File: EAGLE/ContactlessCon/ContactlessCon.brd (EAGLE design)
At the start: 57.1 x 31.4 mm, 5 parts, among them J1 PINHEADER-212*1, J2 PINHEADER-818*1, X1 0446200002

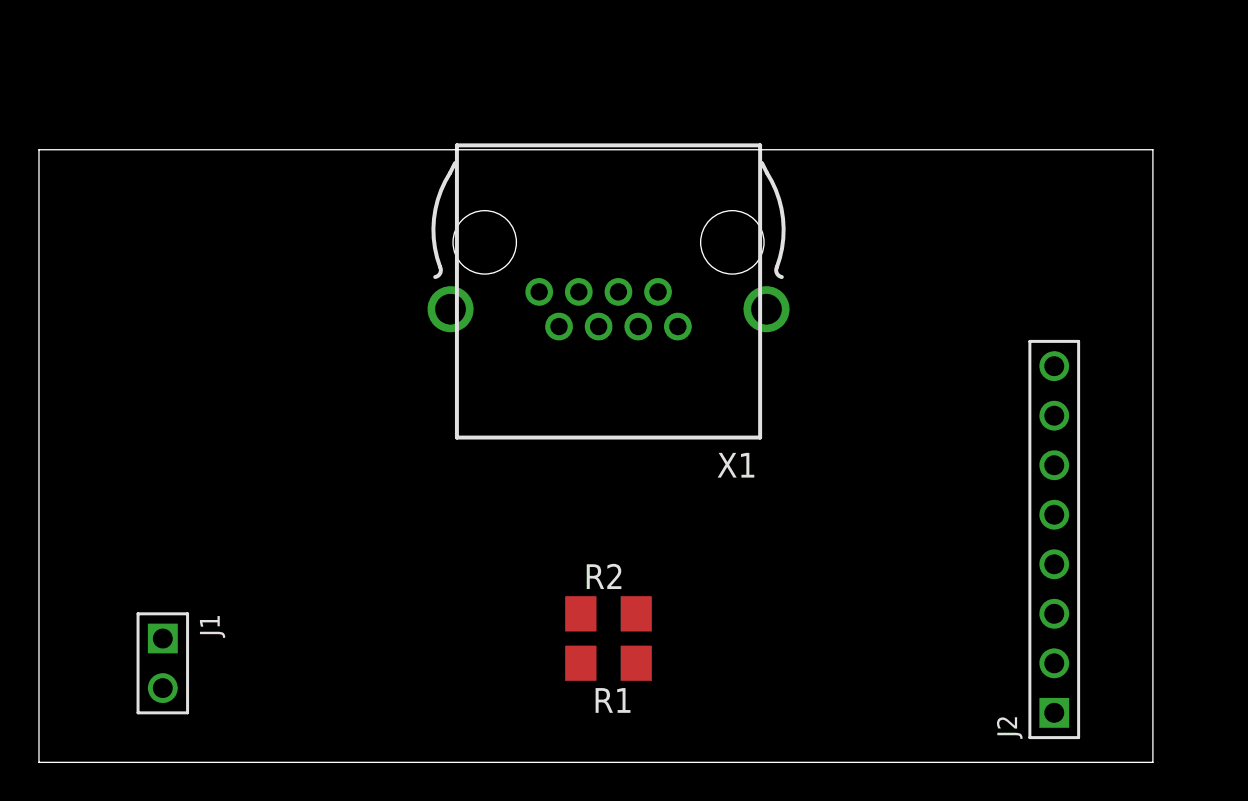
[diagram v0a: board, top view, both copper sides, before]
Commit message: Conの配線終了
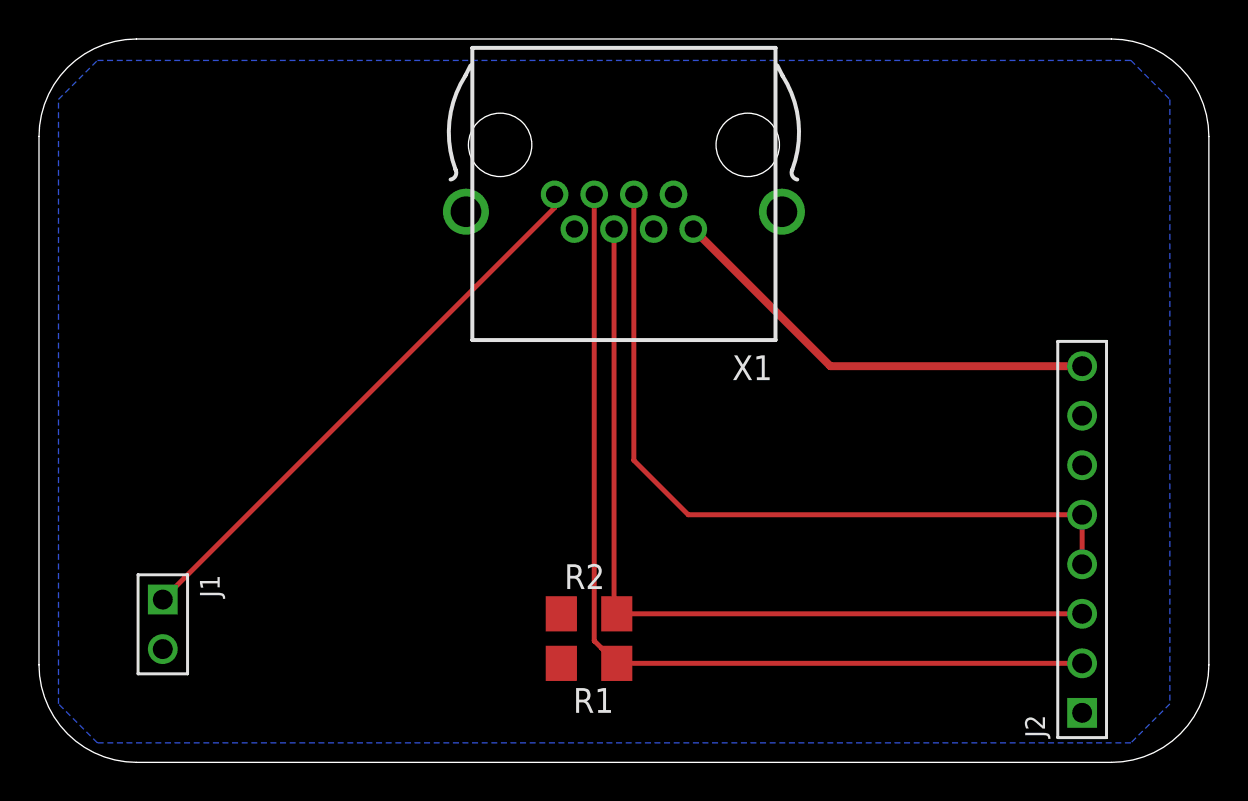
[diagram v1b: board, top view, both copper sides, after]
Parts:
- moved X1 5.06 mm to (30.0, 31.7)
- moved J1 2.00 mm to (6.35, 7.08)
- moved J2 1.43 mm to (53.5, 8.89)
- moved R1 1.00 mm to (28.2, 5.08)
- moved R2 1.00 mm to (28.2, 7.62)
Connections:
- net GPIO: now also X1.5; no longer X1.3
- net SCL: now also X1.4; no longer X1.5
- net SDA: now also X1.3; no longer X1.4
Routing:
- net SDA: track 0.00 -> 48.4 mm
- net SCL: track 0.00 -> 44.0 mm
- net GPIO: track 0.00 -> 40.3 mm
- net SPEAKER: track 0.00 -> 29.1 mm
- net +3V3: track 0.00 -> 22.9 mm
- added copper zone on layer 16, net GND
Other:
- board size 57.1 x 31.4 mm -> 60 x 37.1 mm
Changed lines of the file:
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@@
 <board>
 <plain>
-<wire x1="0" y1="0" x2="57.13" y2="0" width="0" layer="20"/>
-<wire x1="57.13" y1="0" x2="57.13" y2="31.42" width="0" layer="20"/>
-<wire x1="57.13" y1="31.42" x2="0" y2="31.42" width="0" layer="20"/>
-<wire x1="0" y1="31.42" x2="0" y2="0" width="0" layer="20"/>
+<wire x1="0" y1="32.1" x2="0" y2="5" width="0" layer="20"/>
+<wire x1="0" y1="5" x2="5" y2="0" width="0" layer="20" curve="90"/>
+<wire x1="5" y1="0" x2="55" y2="0" width="0" layer="20"/>
+<wire x1="55" y1="0" x2="60" y2="5" width="0" layer="20" curve="90"/>
+<wire x1="60" y1="5" x2="60" y2="32.1" width="0" layer="20"/>
+<wire x1="60" y1="32.1" x2="55" y2="37.1" width="0" layer="20" curve="90"/>
+<wire x1="55" y1="37.1" x2="5" y2="37.1" width="0" layer="20"/>
+<wire x1="5" y1="37.1" x2="0" y2="32.1" width="0" layer="20" curve="90"/>
 </plain>
 <attributes>
@@
 </autorouter>
 <elements>
-<element name="J1" library="PINHEADER" package="PINHEADER-2*1" value="PINHEADER-212*1" x="6.35" y="5.08" smashed="yes" rot="R270">
-<attribute name="NAME" x="8.255" y="7.62" size="1.016" layer="21" font="vector" ratio="15" rot="R270"/>
-</element>
-<element name="J2" library="PINHEADER" package="PINHEADER-8*1" value="PINHEADER-818*1" x="52.07" y="8.89" smashed="yes" rot="R90">
-<attribute name="NAME" x="50.165" y="1.27" size="1.016" layer="25" font="vector" ratio="15" rot="R90"/>
-</element>
-<element name="R1" library="rcl" library_urn="urn:adsk.eagle:library:334" package="R1206" package3d_urn="urn:adsk.eagle:package:23540/2" value="" x="29.21" y="5.08" smashed="yes" rot="R180">
-<attribute name="NAME" x="30.48" y="3.81" size="1.27" layer="25" rot="R180"/>
-<attribute name="POPULARITY" value="41" x="13.97" y="34.29" size="1.778" layer="27" rot="R180" display="off"/>
-<attribute name="SPICEPREFIX" value="R" x="13.97" y="34.29" size="1.778" layer="27" rot="R180" display="off"/>
-<attribute name="VALUE" x="30.48" y="7.62" size="1.27" layer="27" rot="R180"/>
-</element>
-<element name="R2" library="rcl" library_urn="urn:adsk.eagle:library:334" package="R1206" package3d_urn="urn:adsk.eagle:package:23540/2" value="" x="29.21" y="7.62" smashed="yes" rot="R180">
-<attribute name="NAME" x="27.94" y="8.89" size="1.27" layer="25"/>
-<attribute name="POPULARITY" value="41" x="8.89" y="36.83" size="1.778" layer="27" rot="R180" display="off"/>
-<attribute name="SPICEPREFIX" value="R" x="8.89" y="36.83" size="1.778" layer="27" rot="R180" display="off"/>
-<attribute name="VALUE" x="30.48" y="10.16" size="1.27" layer="27" rot="R180"/>
-</element>
-<element name="X1" library="con-molex" library_urn="urn:adsk.eagle:library:165" package="0446200002" package3d_urn="urn:adsk.eagle:package:8078921/1" value="0446200002" x="29.21" y="26.67" smashed="yes" rot="R180">
-<attribute name="MF" value="MOLEX" x="6.35" y="31.75" size="1.778" layer="27" rot="R180" display="off"/>
-<attribute name="MPN" value="0446200002" x="6.35" y="31.75" size="1.778" layer="27" rot="R180" display="off"/>
-<attribute name="NAME" x="36.83" y="15.875" size="1.27" layer="25" rot="R180"/>
-<attribute name="OC_FARNELL" value="9251910" x="6.35" y="31.75" size="1.778" layer="27" rot="R180" display="off"/>
-<attribute name="POPULARITY" value="0" x="6.35" y="31.75" size="1.778" layer="27" rot="R180" display="off"/>
-<attribute name="VALUE" x="35.56" y="19.05" size="1.27" layer="27" rot="R180"/>
+<element name="J1" library="PINHEADER" package="PINHEADER-2*1" value="PINHEADER-212*1" x="6.35" y="7.08" smashed="yes" rot="R270">
+<attribute name="NAME" x="8.255" y="9.62" size="1.016" layer="21" font="vector" ratio="15" rot="R270"/>
+</element>
+<element name="J2" library="PINHEADER" package="PINHEADER-8*1" value="PINHEADER-818*1" x="53.5" y="8.89" smashed="yes" rot="R90">
+<attribute name="NAME" x="51.595" y="1.27" size="1.016" layer="25" font="vector" ratio="15" rot="R90"/>
+</element>
+<element name="R1" library="rcl" library_urn="urn:adsk.eagle:library:334" package="R1206" package3d_urn="urn:adsk.eagle:package:23540/2" value="" x="28.21" y="5.08" smashed="yes" rot="R180">
+<attribute name="NAME" x="29.48" y="3.81" size="1.27" layer="25" rot="R180"/>
+<attribute name="POPULARITY" value="41" x="12.97" y="34.29" size="1.778" layer="27" rot="R180" display="off"/>
+<attribute name="SPICEPREFIX" value="R" x="12.97" y="34.29" size="1.778" layer="27" rot="R180" display="off"/>
+<attribute name="VALUE" x="29.48" y="7.62" size="1.27" layer="27" rot="R180"/>
+</element>
+<element name="R2" library="rcl" library_urn="urn:adsk.eagle:library:334" package="R1206" package3d_urn="urn:adsk.eagle:package:23540/2" value="" x="28.21" y="7.62" smashed="yes" rot="R180">
+<attribute name="NAME" x="26.94" y="8.89" size="1.27" layer="25"/>
+<attribute name="POPULARITY" value="41" x="7.89" y="36.83" size="1.778" layer="27" rot="R180" display="off"/>
+<attribute name="SPICEPREFIX" value="R" x="7.89" y="36.83" size="1.778" layer="27" rot="R180" display="off"/>
+<attribute name="VALUE" x="29.48" y="10.16" size="1.27" layer="27" rot="R180"/>
+</element>
+<element name="X1" library="con-molex" library_urn="urn:adsk.eagle:library:165" package="0446200002" package3d_urn="urn:adsk.eagle:package:8078921/1" value="0446200002" x="30" y="31.67" smashed="yes" rot="R180">
+<attribute name="MF" value="MOLEX" x="7.14" y="36.75" size="1.778" layer="27" rot="R180" display="off"/>
+<attribute name="MPN" value="0446200002" x="7.14" y="36.75" size="1.778" layer="27" rot="R180" display="off"/>
+<attribute name="NAME" x="37.62" y="20.875" size="1.27" layer="25" rot="R180"/>
+<attribute name="OC_FARNELL" value="9251910" x="7.14" y="36.75" size="1.778" layer="27" rot="R180" display="off"/>
+<attribute name="POPULARITY" value="0" x="7.14" y="36.75" size="1.778" layer="27" rot="R180" display="off"/>
+<attribute name="VALUE" x="36.35" y="24.05" size="1.27" layer="27" rot="R180"/>
 </element>
 </elements>
@@
 <contactref element="X1" pad="8"/>
 <contactref element="X1" pad="6"/>
-<wire x1="30.734" y1="22.352" x2="32.766" y2="22.352" width="0" layer="19" extent="1-1"/>
-<wire x1="52.07" y1="20.32" x2="30.734" y2="22.352" width="0" layer="19" extent="1-1"/>
-<wire x1="27.788" y1="5.08" x2="52.07" y2="20.32" width="0" layer="19" extent="1-1"/>
-<wire x1="27.788" y1="7.62" x2="27.788" y2="5.08" width="0" layer="19" extent="1-1"/>
+<wire x1="53.5" y1="20.32" x2="40.588" y2="20.32" width="0.4064" layer="1"/>
+<wire x1="40.588" y1="20.32" x2="33.556" y2="27.352" width="0.4064" layer="1"/>
+<wire x1="31.524" y1="27.352" x2="33.556" y2="27.352" width="0" layer="19" extent="1-1"/>
+<wire x1="26.788" y1="7.62" x2="31.524" y2="27.352" width="0" layer="19" extent="1-1"/>
+<wire x1="26.788" y1="5.08" x2="26.788" y2="7.62" width="0" layer="19" extent="1-1"/>
 </signal>
 <signal name="GND">
@@
 <contactref element="X1" pad="7"/>
 <contactref element="X1" pad="2"/>
-<wire x1="26.67" y1="22.352" x2="31.75" y2="24.13" width="0" layer="19" extent="1-1"/>
-<wire x1="6.35" y1="3.81" x2="26.67" y2="22.352" width="0" layer="19" extent="1-1"/>
-<wire x1="52.07" y1="15.24" x2="6.35" y2="3.81" width="0" layer="19" extent="1-1"/>
-<wire x1="52.07" y1="2.54" x2="52.07" y2="15.24" width="0" layer="19" extent="1-1"/>
+<polygon width="0.127" layer="16" isolate="0.4064">
+<vertex x="3" y="36"/>
+<vertex x="56" y="36"/>
+<vertex x="58" y="34"/>
+<vertex x="58" y="3"/>
+<vertex x="56" y="1"/>
+<vertex x="3" y="1"/>
+<vertex x="1" y="3"/>
+<vertex x="1" y="34"/>
+</polygon>
 </signal>
 <signal name="GPIO">
 <contactref element="J2" pad="5"/>
 <contactref element="J2" pad="4"/>
-<contactref element="X1" pad="3"/>
-<wire x1="52.07" y1="12.7" x2="27.686" y2="24.13" width="0" layer="19" extent="1-1"/>
-<wire x1="52.07" y1="10.16" x2="52.07" y2="12.7" width="0" layer="19" extent="1-1"/>
+<wire x1="53.5" y1="10.16" x2="53.5" y2="12.7" width="0.254" layer="1"/>
+<contactref element="X1" pad="5"/>
+<wire x1="30.508" y1="29.13" x2="30.508" y2="15.492" width="0.254" layer="1"/>
+<wire x1="33.3" y1="12.7" x2="53.5" y2="12.7" width="0.254" layer="1"/>
+<wire x1="30.508" y1="15.492" x2="33.3" y2="12.7" width="0.254" layer="1"/>
 </signal>
 <signal name="SCL">
 <contactref element="J2" pad="3"/>
 <contactref element="R2" pad="1"/>
-<contactref element="X1" pad="5"/>
-<wire x1="52.07" y1="7.62" x2="29.718" y2="24.13" width="0" layer="19" extent="1-1"/>
-<wire x1="30.632" y1="7.62" x2="52.07" y2="7.62" width="0" layer="19" extent="1-1"/>
+<wire x1="29.508" y1="7.744" x2="29.632" y2="7.62" width="0.254" layer="1"/>
+<wire x1="53.5" y1="7.62" x2="30" y2="7.62" width="0.254" layer="1"/>
+<contactref element="X1" pad="4"/>
+<wire x1="30" y1="7.62" x2="29.632" y2="7.62" width="0.254" layer="1"/>
+<wire x1="29.492" y1="27.352" x2="29.492" y2="8.128" width="0.254" layer="1"/>
+<wire x1="29.492" y1="8.128" x2="30" y2="7.62" width="0.254" layer="1"/>
 </signal>
 <signal name="SDA">
 <contactref element="J2" pad="2"/>
 <contactref element="R1" pad="1"/>
-<contactref element="X1" pad="4"/>
-<wire x1="52.07" y1="5.08" x2="30.632" y2="5.08" width="0" layer="19" extent="1-1"/>
-<wire x1="28.702" y1="22.352" x2="52.07" y2="5.08" width="0" layer="19" extent="1-1"/>
+<wire x1="28.492" y1="6.22" x2="28.856" y2="5.856" width="0.254" layer="1"/>
+<wire x1="28.856" y1="5.856" x2="29.632" y2="5.08" width="0.254" layer="1"/>
+<wire x1="29.632" y1="5.08" x2="53.5" y2="5.08" width="0.254" layer="1"/>
+<contactref element="X1" pad="3"/>
+<wire x1="28.476" y1="29.13" x2="28.476" y2="6.236" width="0.254" layer="1"/>
+<wire x1="28.476" y1="6.236" x2="28.492" y2="6.22" width="0.254" layer="1"/>
 </signal>
 <signal name="SPEAKER">
 <contactref element="J1" pad="1"/>
 <contactref element="X1" pad="1"/>
-<wire x1="6.35" y1="6.35" x2="25.654" y2="24.13" width="0" layer="19" extent="1-1"/>
+<wire x1="6.35" y1="8.35" x2="26.444" y2="28.444" width="0.254" layer="1"/>
+<wire x1="26.444" y1="28.444" x2="26.444" y2="29.13" width="0.254" layer="1"/>
 </signal>
 </signals>
